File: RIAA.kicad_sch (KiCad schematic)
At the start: 67 parts, among them K1 G6K-2, P10 From Keyboard, P8 From main PCB, P9 From Wire, U5 OPA2134, U6 OPA2134, U7 LM317_TO-220

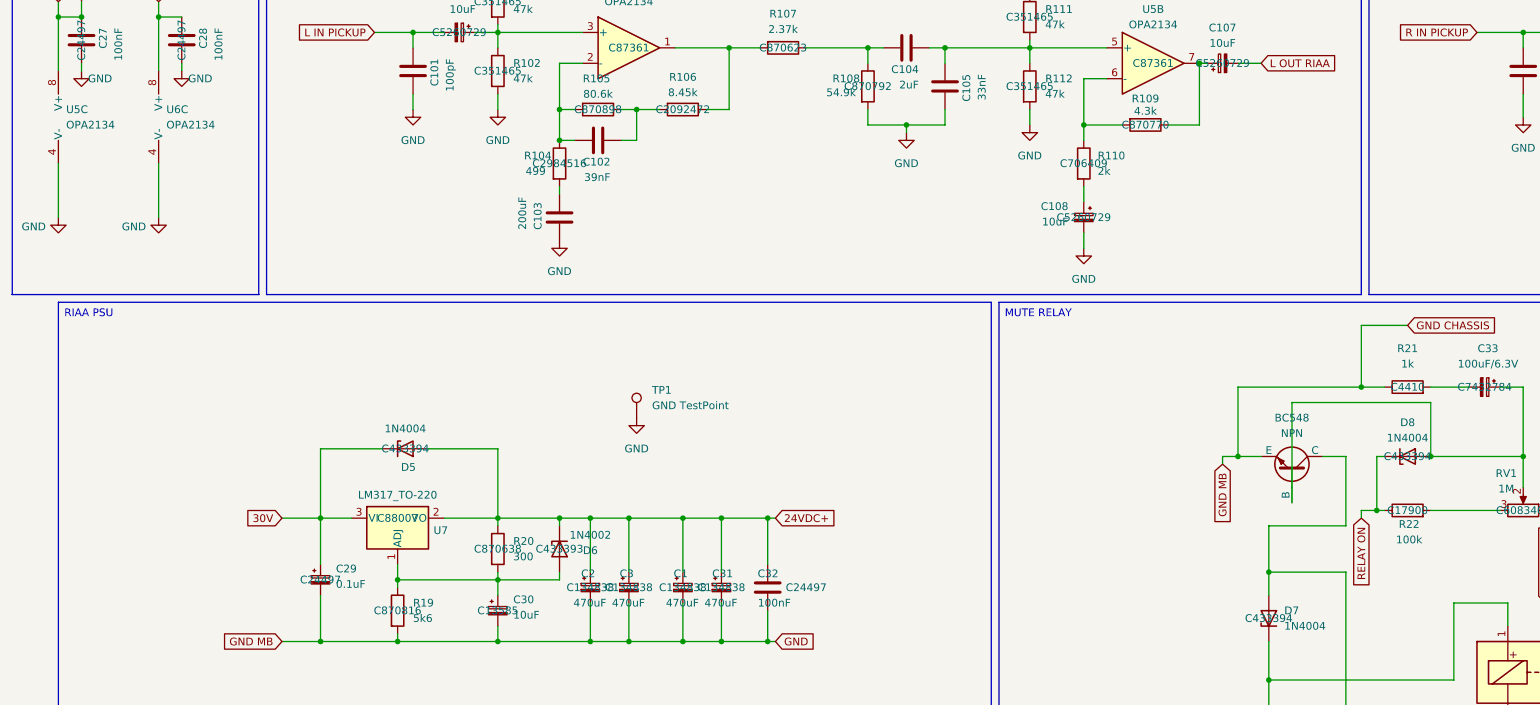
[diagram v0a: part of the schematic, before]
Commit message: WIP: Finishing up SMD version.
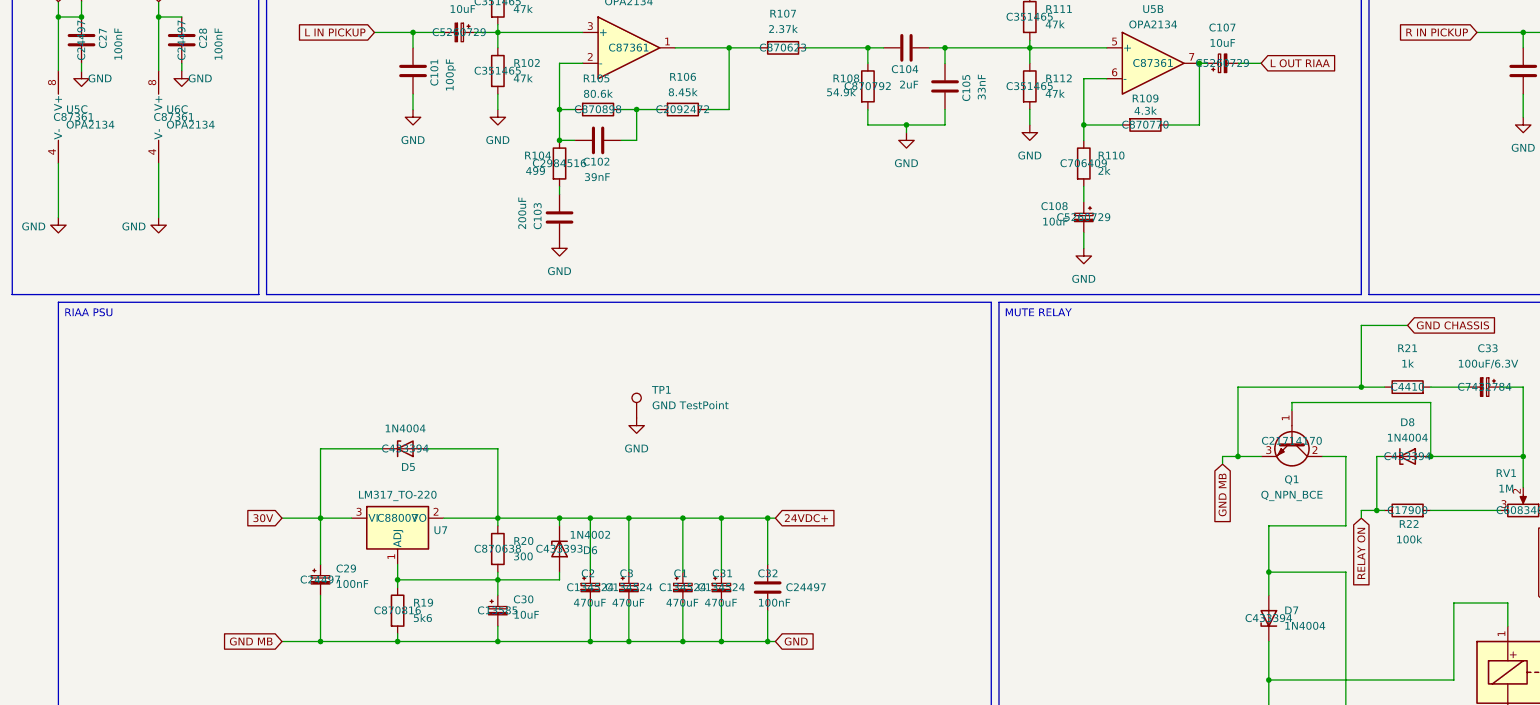
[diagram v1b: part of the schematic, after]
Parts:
- removed BC548: NPN, Package_TO_SOT_SMD:SOT-23_Handsoldering, symbol Simulation_SPICE:NPN
- added Q1: Q_NPN_BCE, Package_TO_SOT_SMD:SOT-89-3_Handsoldering, symbol Transistor_BJT:Q_NPN_BCE
- C1, C2, C3, C31: LCSC PN (none) -> C134524; LSCS PN C134838 -> (none)
- C101, C102, C103, C104, C105, C201, C202, C203, C204, C205, P10, P8, P9, RV1, TP1, TP2: now left out of the parts list
- C106, C107, C108, C206, C207, C208: LCSC PN (none) -> C5260729; LSCS PN C5260729 -> (none)
- C27, C28, C32: LCSC PN (none) -> C24497; LSCS PN C24497 -> (none)
- C29: value 0.1uF -> 100nF; LCSC PN (none) -> C24497; LSCS PN C24497 -> (none)
- C30: LCSC PN (none) -> C13585; LSCS PN C13585 -> (none)
- C33: LCSC PN (none) -> C7432784; LSCS PN C7432784 -> (none)
- D5, D7, D8: LCSC PN (none) -> C433394; LSCS PN C433394 -> (none)
- D6: LCSC PN (none) -> C433393; LSCS PN C433393 -> (none)
- R102, R103, R111, R112, R202, R203, R211, R212: LCSC PN (none) -> C351465; LSCS PN C351465 -> (none)
- R104, R204: LCSC PN (none) -> C2984516; LSCS PN C2984516 -> (none)
- R105, R205: LCSC PN (none) -> C870898; LSCS PN C870898 -> (none)
- R106, R206: LCSC PN (none) -> C2092472; LSCS PN C2092472 -> (none)
- R107, R207: LCSC PN (none) -> C870623; LSCS PN C870623 -> (none)
- R108, R208: LCSC PN (none) -> C870792; LSCS PN C870792 -> (none)
- R109, R209: LCSC PN (none) -> C870770; LSCS PN C870770 -> (none)
- R110, R210: LCSC PN (none) -> C706409; LSCS PN C706409 -> (none)
- R19: LCSC PN (none) -> C870816; LSCS PN C870816 -> (none)
- R20: LCSC PN (none) -> C870638; LSCS PN C870638 -> (none)
- R21: LCSC PN (none) -> C4410; LSCS PN C4410 -> (none)
- R22: LCSC PN (none) -> C17900; LSCS PN C17900 -> (none)
- U5, U6: LCSC PN (none) -> C87361; LSCS PN C87361 -> (none)
- U7: LCSC PN (none) -> C88007; LSCS PN C88007 -> (none)
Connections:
- net GND: now also Q1.3 (E)
- net at D7.2 (A), K1.8: now also Q1.2 (C)
- net at C33.1, D8.2 (A), RV1.2: now also Q1.1 (B)
